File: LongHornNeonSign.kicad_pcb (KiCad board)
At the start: 2 copper layers, 84.5 x 69 mm, 61 parts, among them J1 Screw_Terminal_01x02, J2 Screw_Terminal_01x02, J3 Screw_Terminal_01x02, J4 Screw_Terminal_01x02, Q1 AO3400A, Q2 AO3400A, Q3 AO3400A, Q4 AO3400A, SW1 SW_Push, SW2 SW_Push, SW3 SW_Push, U1 LM2596S-5

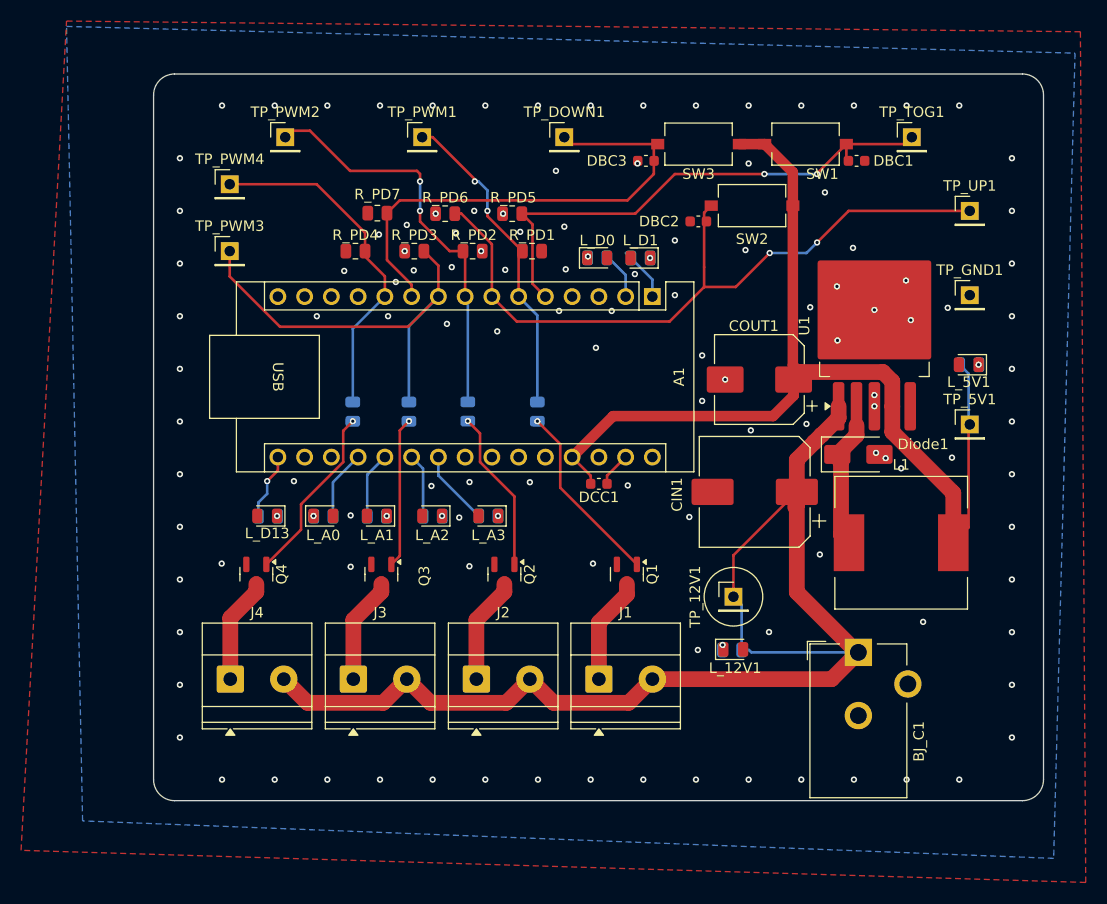
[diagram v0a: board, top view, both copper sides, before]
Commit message: updated pcb
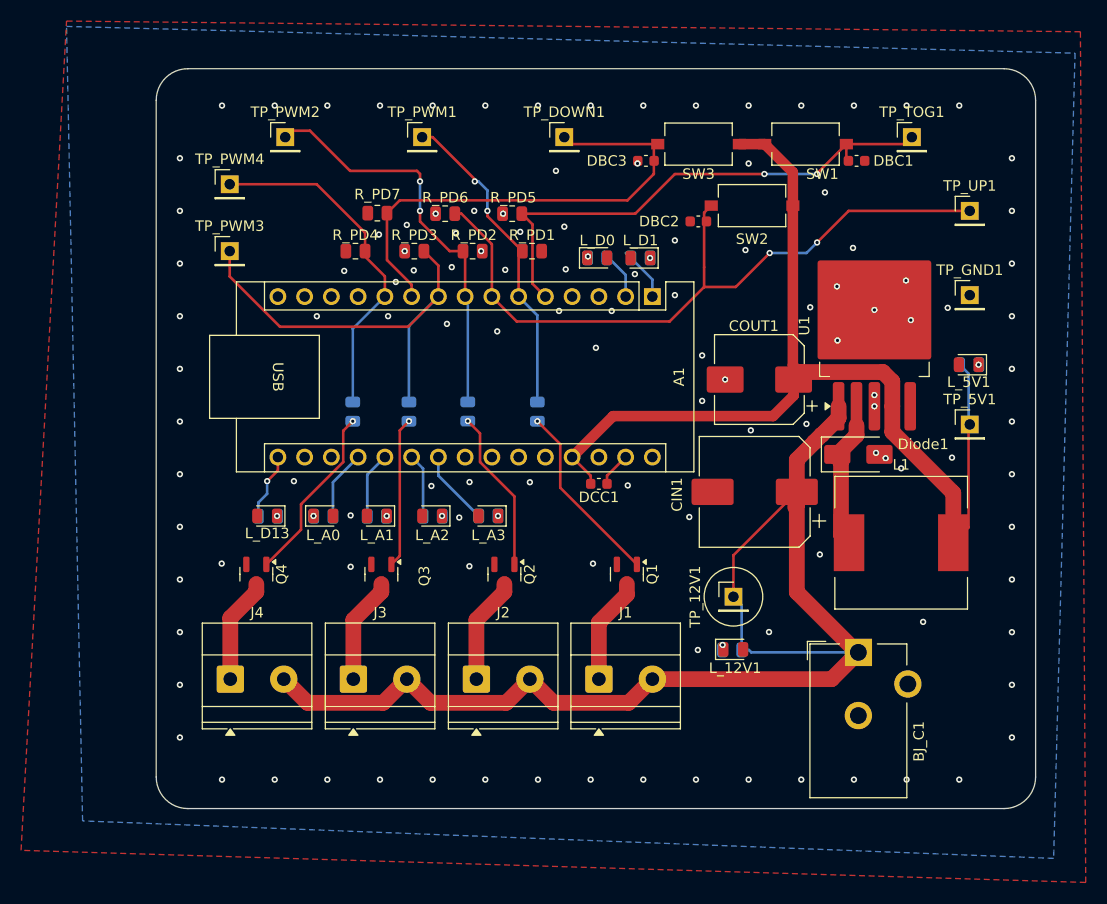
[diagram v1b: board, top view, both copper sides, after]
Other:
- board size 84.5 x 69 mm -> 83.5 x 70.2 mm
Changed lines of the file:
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@@
 	)
 	(gr_line
-		(start 201 136)
-		(end 120.5 136)
+		(start 118.75 133.75)
+		(end 118.75 69.5)
 		(stroke
 			(width 0.05)
@@
 	)
 	(gr_arc
-		(start 201 67)
-		(mid 202.414214 67.585786)
-		(end 203 69)
+		(start 121.75 136.75)
+		(mid 119.62868 135.87132)
+		(end 118.75 133.75)
 		(stroke
 			(width 0.05)
@@
 	)
 	(gr_arc
-		(start 120.5 136)
-		(mid 119.085786 135.414214)
-		(end 118.5 134)
+		(start 199.25 66.5)
+		(mid 201.37132 67.37868)
+		(end 202.25 69.5)
+		(stroke
+			(width 0.05)
+			(type default)
+		)
+		(layer "Edge.Cuts")
+	)
+	(gr_line
+		(start 199.25 136.75)
+		(end 121.75 136.75)
 		(stroke
 			(width 0.05)
@@
 	)
 	(gr_arc
-		(start 203 134)
-		(mid 202.414214 135.414214)
-		(end 201 136)
+		(start 202.25 133.75)
+		(mid 201.37132 135.87132)
+		(end 199.25 136.75)
+		(stroke
+			(width 0.05)
+			(type default)
+		)
+		(layer "Edge.Cuts")
+	)
+	(gr_arc
+		(start 118.75 69.5)
+		(mid 119.62868 67.37868)
+		(end 121.75 66.5)
 		(stroke
 			(width 0.05)
@@
 	)
 	(gr_line
-		(start 118.5 134)
-		(end 118.5 69)
+		(start 121.75 66.5)
+		(end 199.25 66.5)
 		(stroke
 			(width 0.05)
@@
 	)
 	(gr_line
-		(start 203 69)
-		(end 203 134)
+		(start 202.25 69.5)
+		(end 202.25 133.75)
 		(stroke
 			(width 0.05)
-			(type default)
-		)
-		(layer "Edge.Cuts")
-	)
-	(gr_arc
-		(start 118.5 69)
-		(mid 119.085786 67.585786)
-		(end 120.5 67)
-		(stroke
-			(width 0.05)
-			(type default)
-		)
-		(layer "Edge.Cuts")
-	)
-	(gr_line
-		(start 120.5 67)
-		(end 201 67)
-		(stroke
-			(width 0.05)
